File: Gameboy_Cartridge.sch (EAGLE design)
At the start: 3 parts

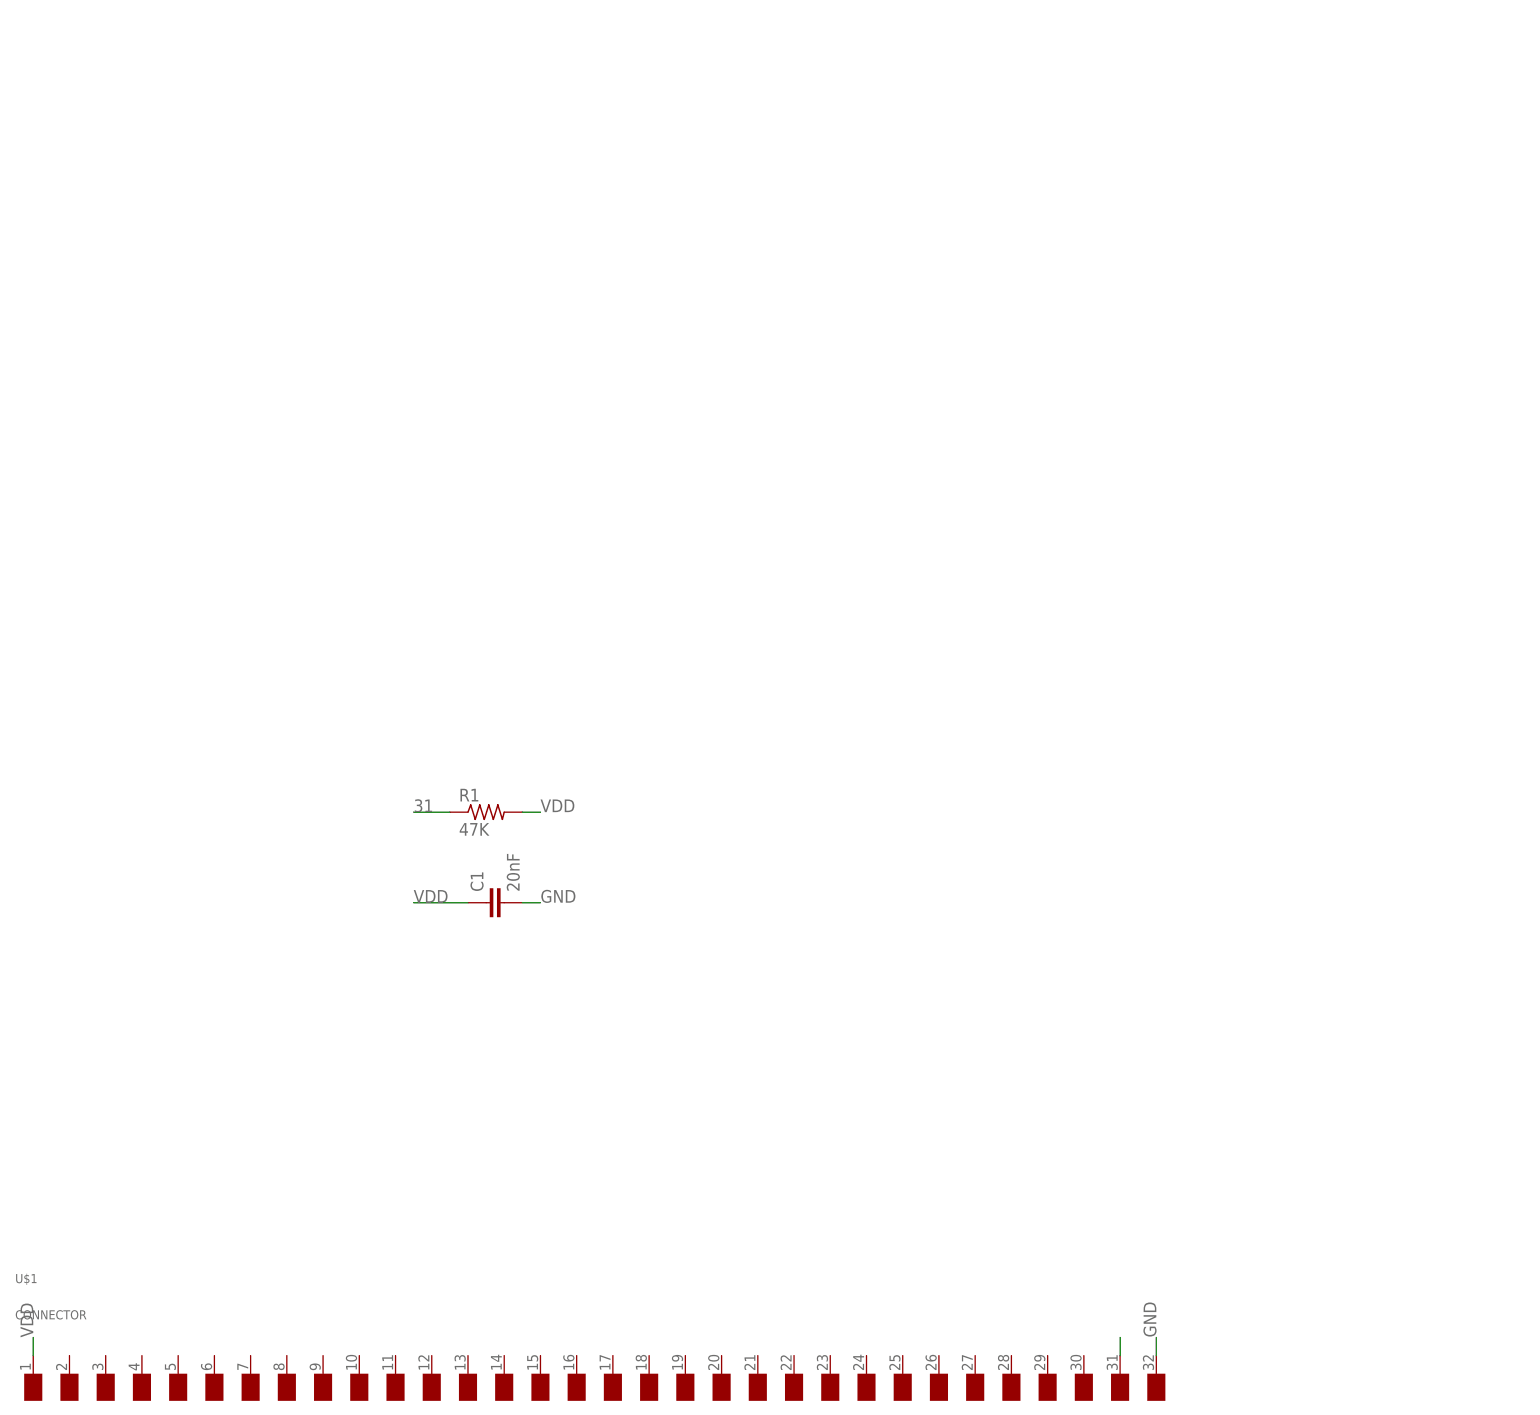
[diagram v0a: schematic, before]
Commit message: add mcu design
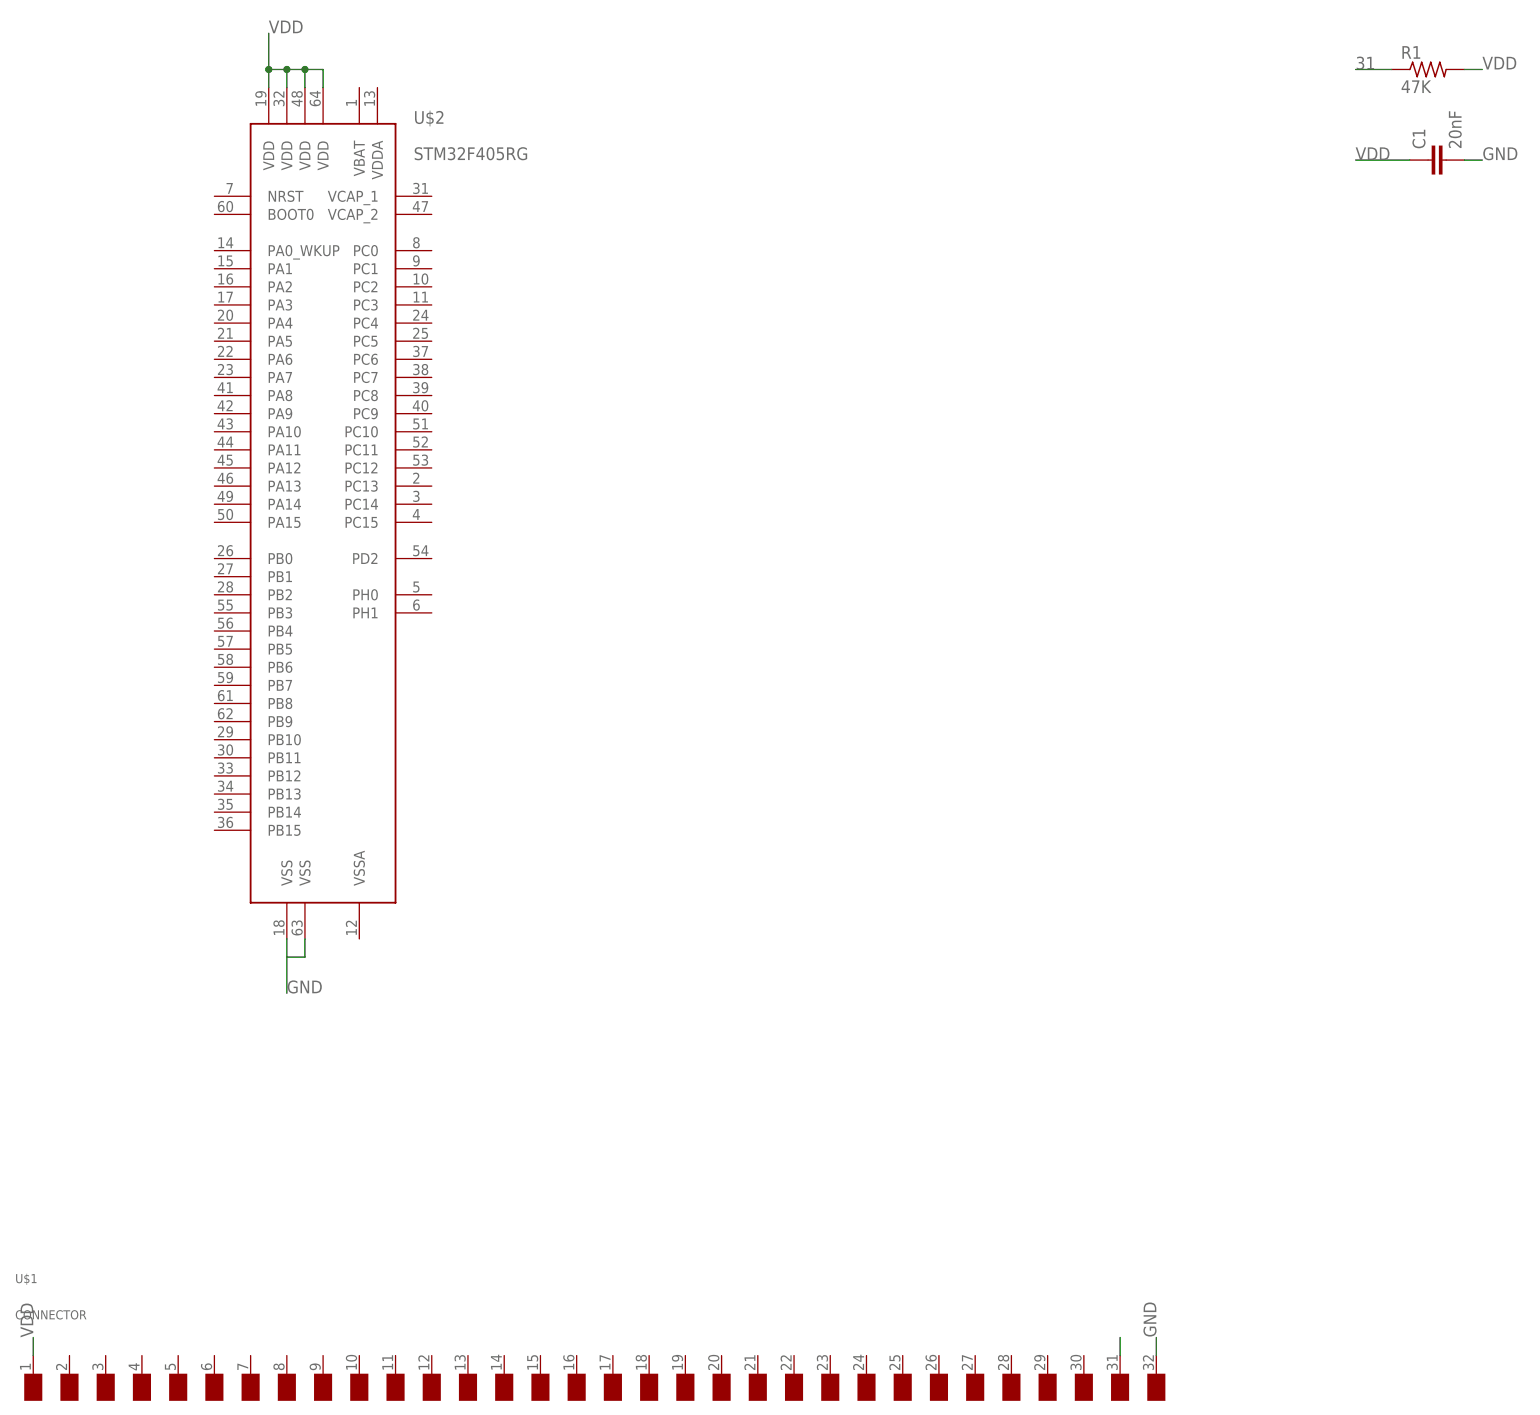
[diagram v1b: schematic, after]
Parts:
- added U$2: STM32F405RG, gameboy:STM32F405RG
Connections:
- new net N$1: U$2.VDD@1, U$2.VDD@2, U$2.VDD@3, U$2.VDD@4
- new net N$2: U$2.VSS@1, U$2.VSS@2
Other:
- moved on the sheet: C1, R1
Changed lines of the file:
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@@
 <?xml version="1.0" encoding="utf-8"?>
 <!DOCTYPE eagle SYSTEM "eagle.dtd">
-<eagle version="7.5.0">
+<eagle version="8.5.1">
 <drawing>
 <settings>
 <setting alwaysvectorfont="no"/>
+<setting keepoldvectorfont="yes"/>
 <setting verticaltext="up"/>
 </settings>
@@
 <part name="R1" library="resistor" deviceset="R-US_" device="M0805" value="47K"/>
 <part name="C1" library="resistor" deviceset="C-EU" device="C0805" value="20nF"/>
+<part name="U$2" library="gameboy" deviceset="STM32F405RG" device=""/>
 </parts>
 <sheets>
@@
 <instances>
 <instance part="U$1" gate="G$1" x="-10.16" y="50.8"/>
-<instance part="R1" gate="G$1" x="55.88" y="129.54"/>
-<instance part="C1" gate="G$1" x="55.88" y="116.84" rot="R90"/>
+<instance part="R1" gate="G$1" x="187.96" y="233.68"/>
+<instance part="C1" gate="G$1" x="187.96" y="220.98" rot="R90"/>
+<instance part="U$2" gate="G$1" x="33.02" y="167.64"/>
 </instances>
 <busses>
@@
 <segment>
 <pinref part="R1" gate="G$1" pin="2"/>
-<wire x1="60.96" y1="129.54" x2="63.5" y2="129.54" width="0.1524" layer="91"/>
-<label x="63.5" y="129.54" size="1.778" layer="95"/>
+<wire x1="193.04" y1="233.68" x2="195.58" y2="233.68" width="0.1524" layer="91"/>
+<label x="195.58" y="233.68" size="1.778" layer="95"/>
+<label x="25.4" y="238.76" size="1.778" layer="95"/>
 </segment>
 <segment>
 <pinref part="C1" gate="G$1" pin="1"/>
-<wire x1="53.34" y1="116.84" x2="45.72" y2="116.84" width="0.1524" layer="91"/>
-<label x="45.72" y="116.84" size="1.778" layer="95"/>
+<wire x1="185.42" y1="220.98" x2="177.8" y2="220.98" width="0.1524" layer="91"/>
+<label x="177.8" y="220.98" size="1.778" layer="95"/>
 </segment>
 </net>
@@
 <segment>
 <pinref part="C1" gate="G$1" pin="2"/>
-<wire x1="60.96" y1="116.84" x2="63.5" y2="116.84" width="0.1524" layer="91"/>
-<label x="63.5" y="116.84" size="1.778" layer="95"/>
+<wire x1="193.04" y1="220.98" x2="195.58" y2="220.98" width="0.1524" layer="91"/>
+<label x="195.58" y="220.98" size="1.778" layer="95"/>
+<label x="27.94" y="104.14" size="1.778" layer="95"/>
 </segment>
 </net>
@@
 <segment>
 <pinref part="R1" gate="G$1" pin="1"/>
-<wire x1="50.8" y1="129.54" x2="45.72" y2="129.54" width="0.1524" layer="91"/>
-<label x="45.72" y="129.54" size="1.778" layer="95"/>
+<wire x1="182.88" y1="233.68" x2="177.8" y2="233.68" width="0.1524" layer="91"/>
+<label x="177.8" y="233.68" size="1.778" layer="95"/>
 </segment>
 </net>
+<net name="N$1" class="0">
+<segment>
+<pinref part="U$2" gate="G$1" pin="VDD@1"/>
+<wire x1="25.4" y1="231.14" x2="25.4" y2="233.68" width="0.1524" layer="91"/>
+<wire x1="25.4" y1="233.68" x2="27.94" y2="233.68" width="0.1524" layer="91"/>
+<pinref part="U$2" gate="G$1" pin="VDD@4"/>
+<wire x1="27.94" y1="233.68" x2="30.48" y2="233.68" width="0.1524" layer="91"/>
+<wire x1="30.48" y1="233.68" x2="33.02" y2="233.68" width="0.1524" layer="91"/>
+<wire x1="33.02" y1="233.68" x2="33.02" y2="231.14" width="0.1524" layer="91"/>
+<pinref part="U$2" gate="G$1" pin="VDD@3"/>
+<wire x1="30.48" y1="231.14" x2="30.48" y2="233.68" width="0.1524" layer="91"/>
+<junction x="30.48" y="233.68"/>
+<pinref part="U$2" gate="G$1" pin="VDD@2"/>
+<wire x1="27.94" y1="231.14" x2="27.94" y2="233.68" width="0.1524" layer="91"/>
+<junction x="27.94" y="233.68"/>
+<wire x1="25.4" y1="233.68" x2="25.4" y2="238.76" width="0.1524" layer="91"/>
+<junction x="25.4" y="233.68"/>
+</segment>
+</net>
+<net name="N$2" class="0">
+<segment>
+<pinref part="U$2" gate="G$1" pin="VSS@1"/>
+<wire x1="27.94" y1="111.76" x2="27.94" y2="109.22" width="0.1524" layer="91"/>
+<wire x1="27.94" y1="109.22" x2="30.48" y2="109.22" width="0.1524" layer="91"/>
+<pinref part="U$2" gate="G$1" pin="VSS@2"/>
+<wire x1="30.48" y1="109.22" x2="30.48" y2="111.76" width="0.1524" layer="91"/>
+<wire x1="27.94" y1="109.22" x2="27.94" y2="104.14" width="0.1524" layer="91"/>
+</segment>
+</net>
